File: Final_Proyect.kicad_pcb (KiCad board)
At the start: 2 copper layers, 66 x 52.5 mm, 77 parts, among them J1 Conn_01x10_Pin, J2 VCC GND TTP223, J4 - +, J5 USB_C, U1 ESP32-S3-WROOM-1, U2 AMS1117-3.3, U3 DRV8870DDA, U4 DRV8870DDA, U5 DRV8870DDA, U6 DRV8870DDA, U7 DRV8870DDA

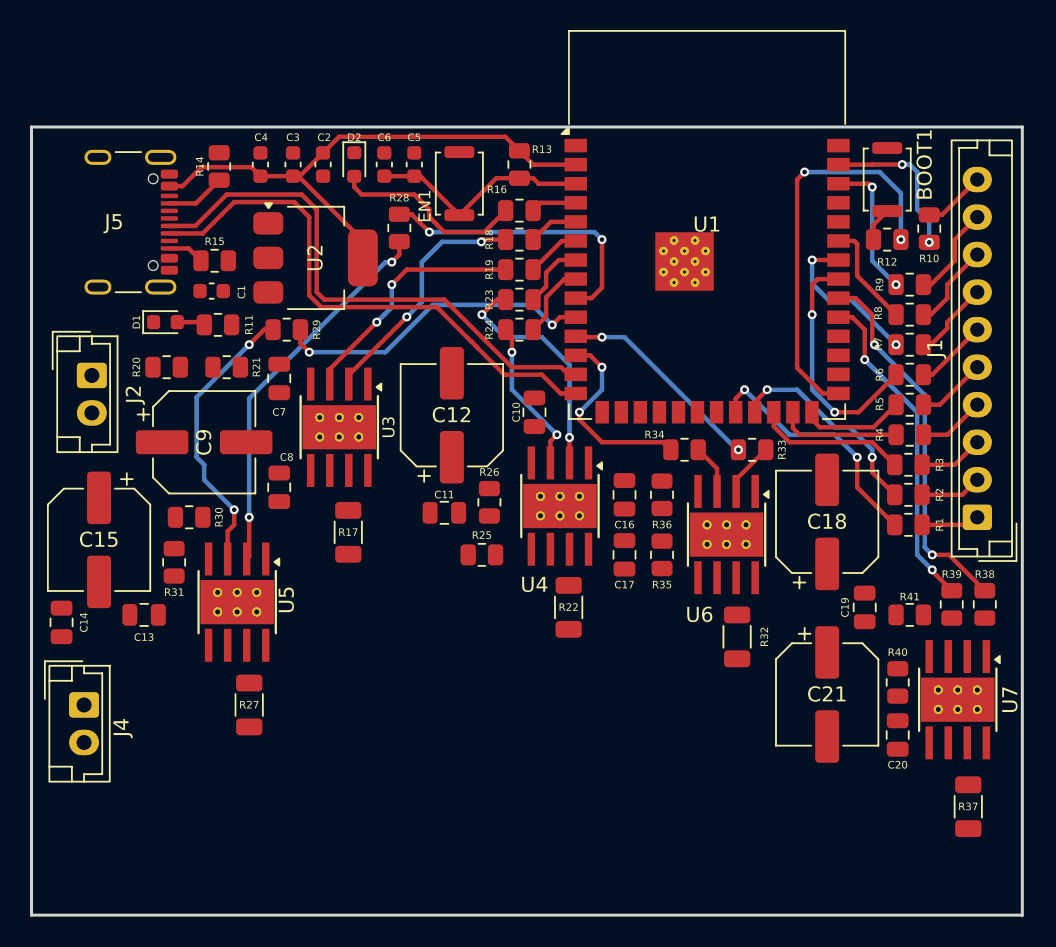
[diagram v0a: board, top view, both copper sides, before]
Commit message: Actualizacion diseño PCB
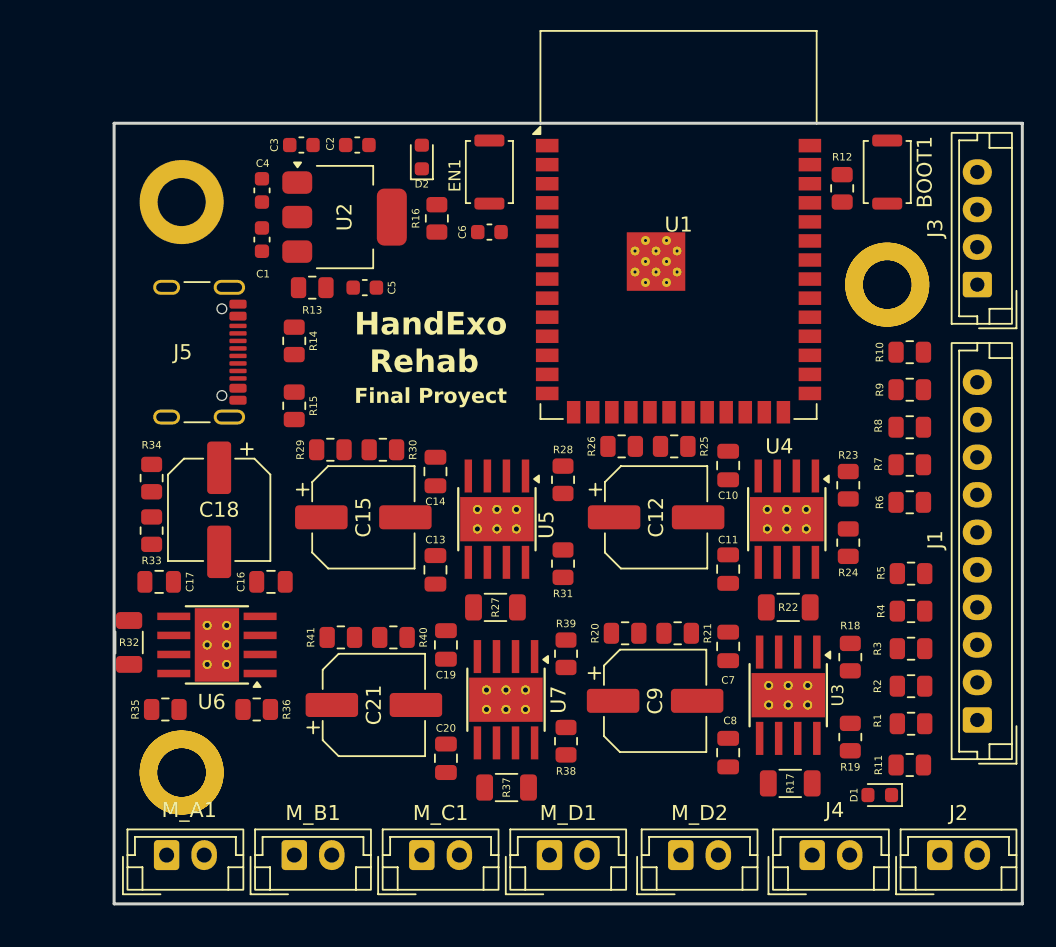
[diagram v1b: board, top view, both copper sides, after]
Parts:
- added ?: , , F.Cu at (158.5, 51.5)
- added ?: , , F.Cu at (111.5, 84.0)
- added J3: OLLED I2C, Connector_JST:JST_EH_B4B-EH-A_1x04_P2.50mm_Vertical, F.Cu at (164.5, 51.5)
- added M_A1: VCC GND TTP223, Connector_JST:JST_EH_B2B-EH-A_1x02_P2.50mm_Vertical, F.Cu at (110.5, 89.5)
- added M_B1: VCC GND TTP223, Connector_JST:JST_EH_B2B-EH-A_1x02_P2.50mm_Vertical, F.Cu at (119.0, 89.5)
- added M_C1: VCC GND TTP223, Connector_JST:JST_EH_B2B-EH-A_1x02_P2.50mm_Vertical, F.Cu at (127.5, 89.5)
- added M_D1: VCC GND TTP223, Connector_JST:JST_EH_B2B-EH-A_1x02_P2.50mm_Vertical, F.Cu at (136.0, 89.5)
- added M_D2: VCC GND TTP223, Connector_JST:JST_EH_B2B-EH-A_1x02_P2.50mm_Vertical, F.Cu at (144.8, 89.5)
- added REF**: MountingHole_3.2mm_M3_DIN965_Pad, MountingHole:MountingHole_3.2mm_M3_DIN965_Pad, F.Cu at (111.5, 46.0)
- added REF**: MountingHole_3.2mm_M3_DIN965_Pad, MountingHole:MountingHole_3.2mm_M3_DIN965_Pad, F.Cu at (158.5, 51.5)
- added REF**: MountingHole_3.2mm_M3_DIN965_Pad, MountingHole:MountingHole_3.2mm_M3_DIN965_Pad, F.Cu at (111.5, 84.0)
- moved J2 64.9 mm to (162.0, 89.5), turned to 0 degrees
- moved D1 57.1 mm to (158.0, 85.5), turned to 180 degrees
- moved R11 54.6 mm to (160.0, 83.5), turned to 180 degrees
- moved J4 49.5 mm to (153.5, 89.5), turned to 0 degrees
- moved C18 40.5 mm to (114.0, 66.5), turned to -90 degrees
- moved R32 40.5 mm to (108.0, 75.3)
- moved R33 40.4 mm to (109.5, 67.9), turned to -90 degrees
- moved R19 38.1 mm to (156.0, 81.6), turned to 90 degrees
- moved R41 37.9 mm to (122.1, 75.0)
- moved R34 35.6 mm to (109.5, 64.4), turned to 90 degrees
- moved R18 35.5 mm to (156.0, 76.3), turned to -90 degrees
- moved R20 35.3 mm to (141.0, 74.7)
- moved R21 34.9 mm to (144.5, 74.7)
- moved C7 34.8 mm to (147.9, 75.6)
- moved U3 34.8 mm to (151.9, 78.8)
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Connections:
- U3 pad 6: /Motor Driver/M1 -> /M1
- U3 pad 8: /Motor Driver/M2 -> /M2
- U4 pad 6: /Motor Driver1/M1 -> /M3
- U4 pad 8: /Motor Driver1/M2 -> /M4
- U5 pad 6: /Motor Driver2/M1 -> /M5
- U5 pad 8: /Motor Driver2/M2 -> /M6
- U6 pad 6: /Motor Driver3/M1 -> /M7
- U6 pad 8: /Motor Driver3/M2 -> /M8
- U7 pad 6: /Motor Driver4/M1 -> /M9
- U7 pad 8: /Motor Driver4/M2 -> /M10
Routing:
- net +3V3: track 37.3 -> 0.00 mm
- net D+: track 36.3 -> 0.00 mm
- net D-: track 35.6 -> 0.00 mm
- net BOOT: track 26.8 -> 0.00 mm, vias 2 -> 0
- net /Motor Driver2/IN2: track 25.6 -> 0.00 mm, vias 2 -> 0
- net F+: track 24.9 -> 0.00 mm, vias 2 -> 0
- net F-: track 21.9 -> 0.00 mm, vias 2 -> 0
- net C-: track 21.6 -> 0.00 mm, vias 2 -> 0
- net C+: track 19.4 -> 0.00 mm, vias 2 -> 0
- net /Motor Driver2/IN1: track 18.9 -> 0.00 mm, vias 2 -> 0
- net SIG10: track 16.6 -> 0.00 mm, vias 2 -> 0
- net /Motor Driver/IN2: track 16.3 -> 0.00 mm, vias 2 -> 0
- net /Motor Driver/IN1: track 16.3 -> 0.00 mm, vias 2 -> 0
- net SIG5: track 16.1 -> 0.00 mm, vias 2 -> 0
- net /Motor Driver1/IN2: track 15.8 -> 0.00 mm, vias 2 -> 0
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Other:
- board size 66 x 52.5 mm -> 60.5 x 52 mm
- board text added: "Final Proyect"
- board text added: "HandExo"
- board text added: "Rehab"
